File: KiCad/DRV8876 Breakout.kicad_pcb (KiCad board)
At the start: 2 copper layers, 40.6 x 40.6 mm, 12 parts, among them J1 Conn_01x08, J2 Conn_01x08, U1 DRV8876

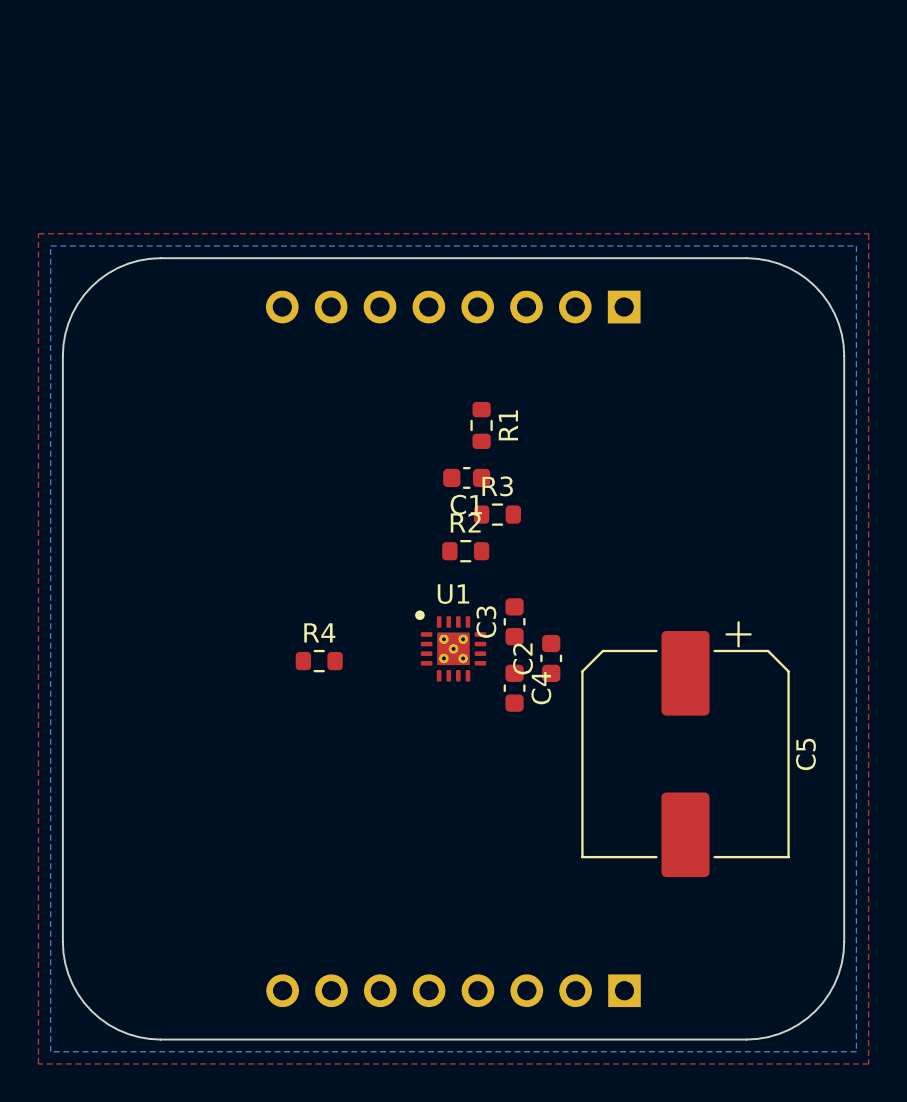
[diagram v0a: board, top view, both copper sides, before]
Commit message: Finished Schematic and PCB
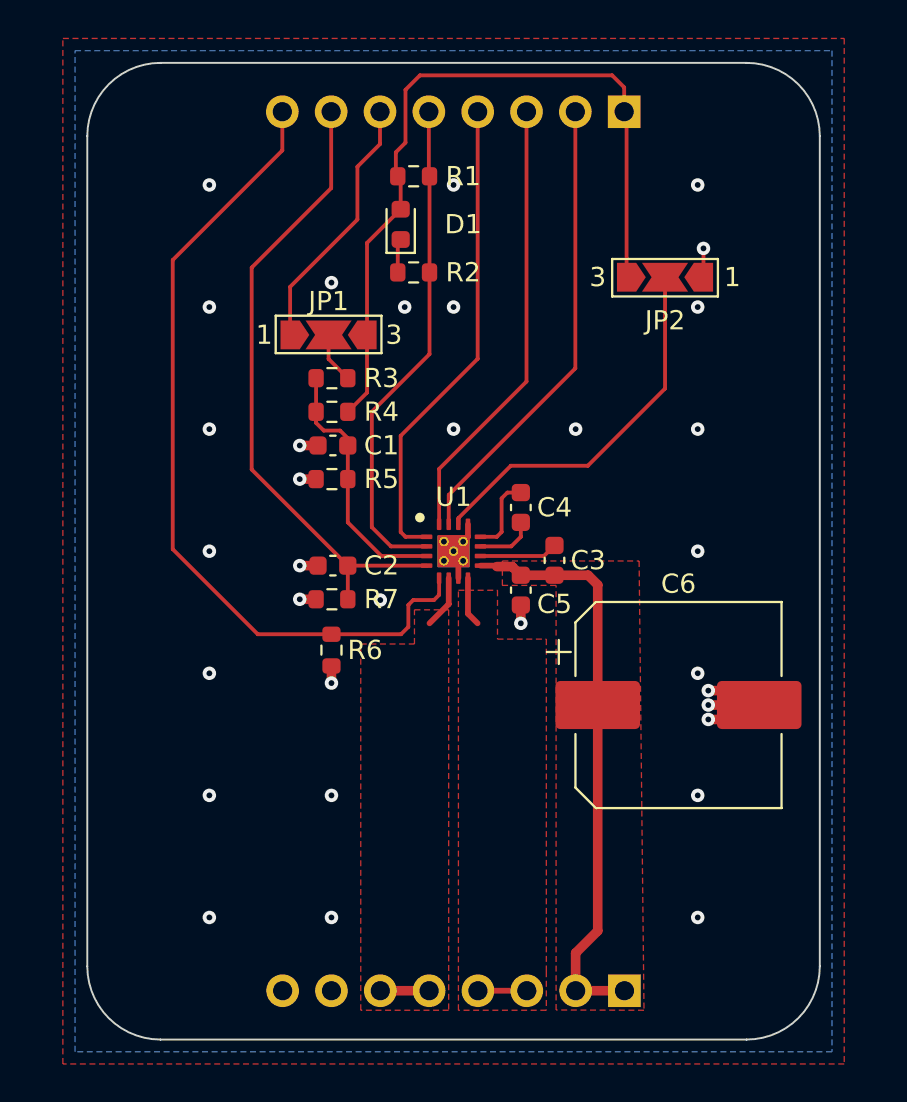
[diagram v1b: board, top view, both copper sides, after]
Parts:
- added C6: 470uF, Capacitor_SMD:CP_Elec_10x10.5, F.Cu at (159.0, 89.3)
- added D1: KT-0603W White, LED_SMD:LED_0603_1608Metric, F.Cu at (144.6, 64.3)
- added JP1: Vref Jumper, Jumper:SolderJumper-3_P2.0mm_Open_TrianglePad1.0x1.5mm_NumberLabels, F.Cu at (140.8, 70.0)
- added JP2: PMODE Jumper, Jumper:SolderJumper-3_P2.0mm_Open_TrianglePad1.0x1.5mm_NumberLabels, F.Cu at (158.3, 67.0)
- added R5: R_Small, Resistor_SMD:R_0603_1608Metric, F.Cu at (141.0, 77.5)
- added R6: 0R, Resistor_SMD:R_0603_1608Metric, F.Cu at (141.0, 86.4)
- added R7: 1k6, Resistor_SMD:R_0603_1608Metric, F.Cu at (141.0, 83.8)
- C2, C4: value 100nF -> 22nF
- C3: value 22nF -> 100nF
- C5: value 470uF -> 100nF; footprint Capacitor_SMD:CP_Elec_10x10.5 -> Capacitor_SMD:C_0603_1608Metric
- R2: value R_Small -> 1k
- R3: value R_Small -> 10k
- moved R2 14.8 mm to (145.2, 66.8)
- moved R1 13.4 mm to (145.2, 61.8), turned to 0 degrees
- moved R4 13.0 mm to (141.0, 74.0), turned to 180 degrees
- moved C2 12.3 mm to (141.0, 82.0), turned to 180 degrees
- moved C5 12.1 mm to (150.8, 83.3)
- moved R3 11.2 mm to (141.0, 72.3), turned to 180 degrees
- moved J1 10.2 mm to (156.2, 58.4)
- moved C4 9.41 mm to (150.8, 79.0), turned to 90 degrees
- moved C1 7.16 mm to (141.0, 75.8)
- moved U1 5.08 mm to (147.3, 81.3)
- moved C3 3.81 mm to (152.6, 81.8)
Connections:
- C2 pad 1: /VM -> /IPROPI
- C2 pad 2: Net-(C2-Pad2) -> GND
- C3 pad 1: Net-(C3-Pad1) -> /VM
- C3 pad 2: Net-(C3-Pad2) -> /VCP
- C4 pad 1: /VM -> /CPH
- C4 pad 2: GND -> /CPL
- J1 pad 1: unconnected-(J1-Pad1) -> +3V3
- J1 pad 2: unconnected-(J1-Pad2) -> /EN/IN1
- J1 pad 3: unconnected-(J1-Pad3) -> /PH/IN2
- J1 pad 4: unconnected-(J1-Pad4) -> /nSLEEP
- J1 pad 5: unconnected-(J1-Pad5) -> /nFAULT
- J1 pad 6: unconnected-(J1-Pad6) -> /VREF DAC In
- J1 pad 7: unconnected-(J1-Pad7) -> /IPROPI
- J1 pad 8: unconnected-(J1-Pad8) -> /IMODE
- R1 pad 1: unconnected-(R1-Pad1) -> +3V3
- R1 pad 2: /VREF -> /nFAULT
- R2 pad 1: /VM -> /LED K
- R2 pad 2: /VREF -> /nFAULT
- R3 pad 1: /VREF -> /VREF Jumper
- R3 pad 2: GND -> /VREF
- R4 pad 1: unconnected-(R4-Pad1) -> +3V3
- R4 pad 2: unconnected-(R4-Pad2) -> /VREF
- U1 pad 1: unconnected-(U1-Pad1) -> /nSLEEP
- U1 pad 10: Net-(C2-Pad2) -> /VCP
- U1 pad 11: Net-(C3-Pad1) -> /CPH
- U1 pad 12: Net-(C3-Pad2) -> /CPL
- U1 pad 14: unconnected-(U1-Pad14) -> /PMODE
- U1 pad 15: unconnected-(U1-Pad15) -> /EN/IN1
- U1 pad 16: unconnected-(U1-Pad16) -> /PH/IN2
- U1 pad 2: unconnected-(U1-Pad2) -> /nFAULT
- U1 pad 3: unconnected-(U1-Pad3) -> /VREF
- U1 pad 4: unconnected-(U1-Pad4) -> /IPROPI
- U1 pad 5: unconnected-(U1-Pad5) -> /IMODE
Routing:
- net /IMODE: track 0.00 -> 43.2 mm
- net +3V3: track 0.00 -> 40.1 mm
- net /IPROPI: track 0.00 -> 33.2 mm
- net /VM: track 0.00 -> 30.6 mm
- net /nFAULT: track 0.00 -> 26.1 mm
- net /nSLEEP: track 0.00 -> 25.0 mm
- net /EN/IN1: track 0.00 -> 24.2 mm
- net /PH/IN2: track 0.00 -> 23.3 mm
- net /PMODE: track 0.00 -> 19.6 mm
- net GND: track 0.00 -> 18.8 mm, vias 0 -> 33
- net /VREF DAC In: track 0.00 -> 13.5 mm
- net /VREF: track 0.00 -> 13.5 mm
- net /OUT2: track 0.00 -> 5.30 mm
- net /OUT1: track 0.00 -> 5.10 mm
- net /VCP: track 0.00 -> 4.08 mm
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- added copper zone on F.Cu, net /OUT1
- added copper zone on F.Cu, net /OUT2
- added copper zone on F.Cu, net /VM
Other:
- board size 40.6 x 40.6 mm -> 38.1 x 50.8 mm
